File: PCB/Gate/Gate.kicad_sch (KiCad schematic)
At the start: 424 parts, among them J1 Conn_01x03, J2 Conn_01x03, U1 QR

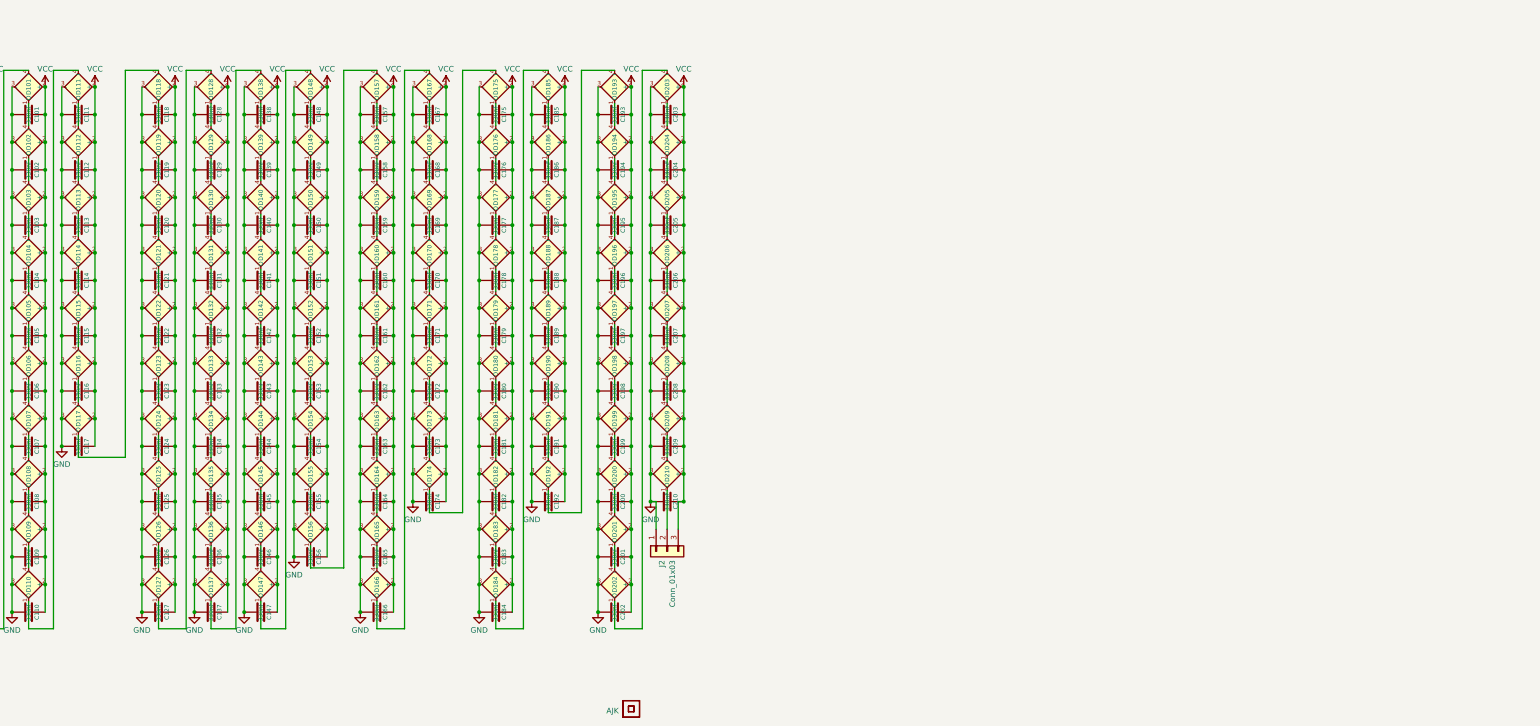
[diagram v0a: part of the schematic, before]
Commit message: Redone
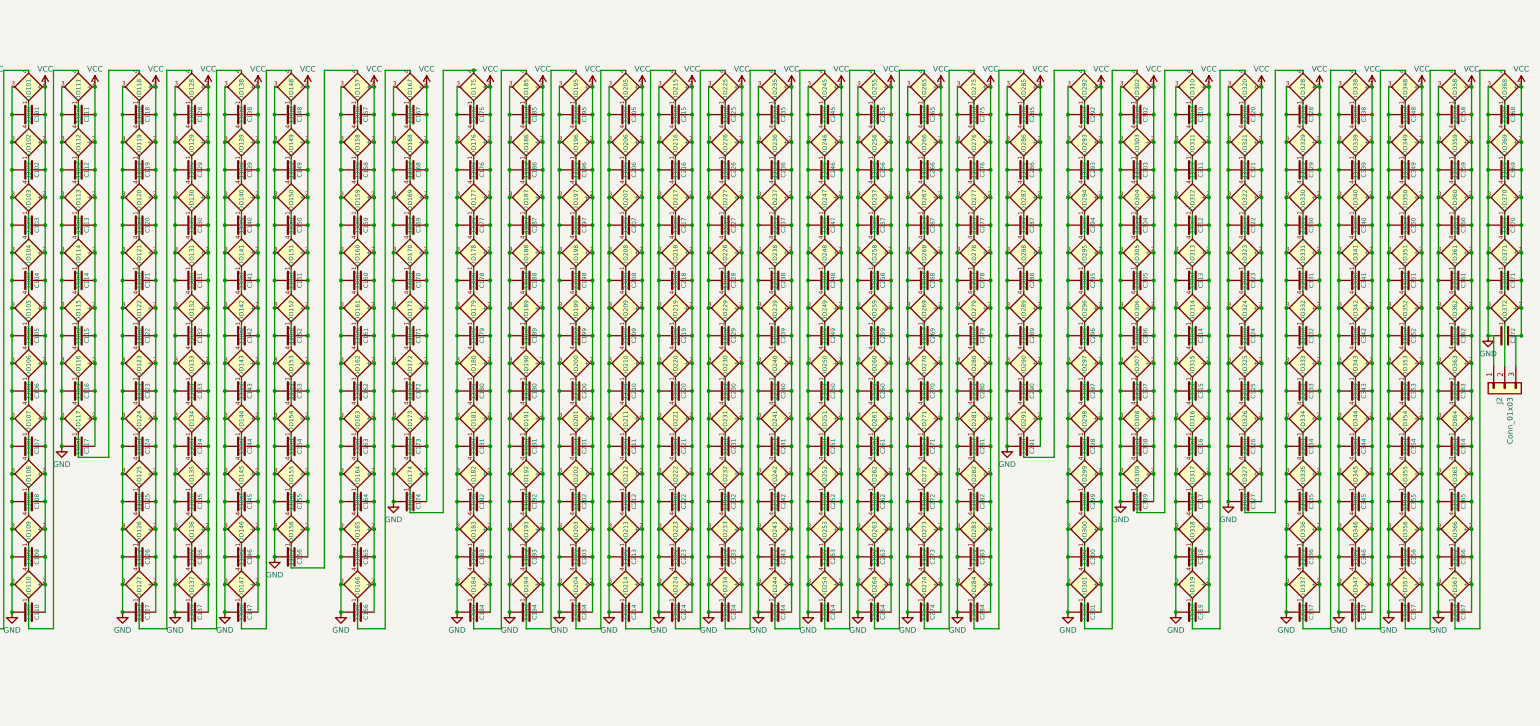
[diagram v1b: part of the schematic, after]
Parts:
- removed Logo1: AJK, RevK:AJK, symbol RevK:AJK
- removed U1: QR, RevK:QR-LED, symbol RevK:QR
- added C211, C212, C213, C214, C215, C216, C217, C218, C219, C220, C221, C222, C223, C224, C225, C226, C227, C228, C229, C230, C231, C232, C233, C234, C235, C236, C237, C238, C239, C240, C241, C242, C243, C244, C245, C246, C247, C248, C249, C250, C251, C252, C253, C254, C255, C256, C257, C258, C259, C260, C261, C262, C263, C264, C265, C266, C267, C268, C269, C270, C271, C272, C273, C274, C275, C276, C277, C278, C279, C280, C281, C282, C283, C284, C285, C286, C287, C288, C289, C290, C291, C292, C293, C294, C295, C296, C297, C298, C299, C300, C301, C302, C303, C304, C305, C306, C307, C308, C309, C310, C311, C312, C313, C314, C315, C316, C317, C318, C319, C320, C321, C322, C323, C324, C325, C326, C327, C328, C329, C330, C331, C332, C333, C334, C335, C336, C337, C338, C339, C340, C341, C342, C343, C344, C345, C346, C347, C348, C349, C350, C351, C352, C353, C354, C355, C356, C357, C358, C359, C360, C361, C362, C363, C364, C365, C366, C367, C368, C369, C370, C371, C372: 330nF, RevK:C_0402, symbol Device:C
- added D211, D212, D213, D214, D215, D216, D217, D218, D219, D220, D221, D222, D223, D224, D225, D226, D227, D228, D229, D230, D231, D232, D233, D234, D235, D236, D237, D238, D239, D240, D241, D242, D243, D244, D245, D246, D247, D248, D249, D250, D251, D252, D253, D254, D255, D256, D257, D258, D259, D260, D261, D262, D263, D264, D265, D266, D267, D268, D269, D270, D271, D272, D273, D274, D275, D276, D277, D278, D279, D280, D281, D282, D283, D284, D285, D286, D287, D288, D289, D290, D291, D292, D293, D294, D295, D296, D297, D298, D299, D300, D301, D302, D303, D304, D305, D306, D307, D308, D309, D310, D311, D312, D313, D314, D315, D316, D317, D318, D319, D320, D321, D322, D323, D324, D325, D326, D327, D328, D329, D330, D331, D332, D333, D334, D335, D336, D337, D338, D339, D340, D341, D342, D343, D344, D345, D346, D347, D348, D349, D350, D351, D352, D353, D354, D355, D356, D357, D358, D359, D360, D361, D362, D363, D364, D365, D366, D367, D368, D369, D370, D371, D372: XL-1010RGBC-WS2812B, RevK:SMD1010, symbol RevK:WS2812B-1mm
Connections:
- net GND: now also C211.2, C212.2, C213.2, C214.2, C215.2, C216.2, C217.2, C218.2, C219.2, C220.2, C221.2, C222.2, C223.2, C224.2, C225.2, C226.2, C227.2, C228.2, C229.2, C230.2, C231.2, C232.2, C233.2, C234.2, C235.2, C236.2, C237.2, C238.2, C239.2, C240.2, C241.2, C242.2, C243.2, C244.2, C245.2, C246.2, C247.2, C248.2, C249.2, C250.2, C251.2, C252.2, C253.2, C254.2, C255.2, C256.2, C257.2, C258.2, C259.2, C260.2, C261.2, C262.2, C263.2, C264.2, C265.2, C266.2, C267.2, C268.2, C269.2, C270.2, C271.2, C272.2, C273.2, C274.2, C275.2, C276.2, C277.2, C278.2, C279.2, C280.2, C281.2, C282.2, C283.2, C284.2, C285.2, C286.2, C287.2, C288.2, C289.2, C290.2, C291.2, C292.2, C293.2, C294.2, C295.2, C296.2, C297.2, C298.2, C299.2, C300.2, C301.2, C302.2, C303.2, C304.2, C305.2, C306.2, C307.2, C308.2, C309.2, C310.2, C311.2, C312.2, C313.2, C314.2, C315.2, C316.2, C317.2, C318.2, C319.2, C320.2, C321.2, C322.2, C323.2, C324.2, C325.2, C326.2, C327.2, C328.2, C329.2, C330.2, C331.2, C332.2, C333.2, C334.2, C335.2, C336.2, C337.2, C338.2, C339.2, C340.2, C341.2, C342.2, C343.2, C344.2, C345.2, C346.2, C347.2, C348.2, C349.2, C350.2, C351.2, C352.2, C353.2, C354.2, C355.2, C356.2, C357.2, C358.2, C359.2, C360.2, C361.2, C362.2, C363.2, C364.2, C365.2, C366.2, C367.2, C368.2, C369.2, C370.2, C371.2, C372.2, D211.3 (-), D212.3 (-), D213.3 (-), D214.3 (-), D215.3 (-), D216.3 (-), D217.3 (-), D218.3 (-), D219.3 (-), D220.3 (-), D221.3 (-), D222.3 (-), D223.3 (-), D224.3 (-), D225.3 (-), D226.3 (-), D227.3 (-), D228.3 (-), D229.3 (-), D230.3 (-), D231.3 (-), D232.3 (-), D233.3 (-), D234.3 (-), D235.3 (-), D236.3 (-), D237.3 (-), D238.3 (-), D239.3 (-), D240.3 (-), D241.3 (-), D242.3 (-), D243.3 (-), D244.3 (-), D245.3 (-), D246.3 (-), D247.3 (-), D248.3 (-), D249.3 (-), D250.3 (-), D251.3 (-), D252.3 (-), D253.3 (-), D254.3 (-), D255.3 (-), D256.3 (-), D257.3 (-), D258.3 (-), D259.3 (-), D260.3 (-), D261.3 (-), D262.3 (-), D263.3 (-), D264.3 (-), D265.3 (-), D266.3 (-), D267.3 (-), D268.3 (-), D269.3 (-), D270.3 (-), D271.3 (-), D272.3 (-), D273.3 (-), D274.3 (-), D275.3 (-), D276.3 (-), D277.3 (-), D278.3 (-), D279.3 (-), D280.3 (-), D281.3 (-), D282.3 (-), D283.3 (-), D284.3 (-), D285.3 (-), D286.3 (-), D287.3 (-), D288.3 (-), D289.3 (-), D290.3 (-), D291.3 (-), D292.3 (-), D293.3 (-), D294.3 (-), D295.3 (-), D296.3 (-), D297.3 (-), D298.3 (-), D299.3 (-), D300.3 (-), D301.3 (-), D302.3 (-), D303.3 (-), D304.3 (-), D305.3 (-), D306.3 (-), D307.3 (-), D308.3 (-), D309.3 (-), D310.3 (-), D311.3 (-), D312.3 (-), D313.3 (-), D314.3 (-), D315.3 (-), D316.3 (-), D317.3 (-), D318.3 (-), D319.3 (-), D320.3 (-), D321.3 (-), D322.3 (-), D323.3 (-), D324.3 (-), D325.3 (-), D326.3 (-), D327.3 (-), D328.3 (-), D329.3 (-), D330.3 (-), D331.3 (-), D332.3 (-), D333.3 (-), D334.3 (-), D335.3 (-), D336.3 (-), D337.3 (-), D338.3 (-), D339.3 (-), D340.3 (-), D341.3 (-), D342.3 (-), D343.3 (-), D344.3 (-), D345.3 (-), D346.3 (-), D347.3 (-), D348.3 (-), D349.3 (-), D350.3 (-), D351.3 (-), D352.3 (-), D353.3 (-), D354.3 (-), D355.3 (-), D356.3 (-), D357.3 (-), D358.3 (-), D359.3 (-), D360.3 (-), D361.3 (-), D362.3 (-), D363.3 (-), D364.3 (-), D365.3 (-), D366.3 (-), D367.3 (-), D368.3 (-), D369.3 (-), D370.3 (-), D371.3 (-), D372.3 (-)
- net VCC: now also C211.1, C212.1, C213.1, C214.1, C215.1, C216.1, C217.1, C218.1, C219.1, C220.1, C221.1, C222.1, C223.1, C224.1, C225.1, C226.1, C227.1, C228.1, C229.1, C230.1, C231.1, C232.1, C233.1, C234.1, C235.1, C236.1, C237.1, C238.1, C239.1, C240.1, C241.1, C242.1, C243.1, C244.1, C245.1, C246.1, C247.1, C248.1, C249.1, C250.1, C251.1, C252.1, C253.1, C254.1, C255.1, C256.1, C257.1, C258.1, C259.1, C260.1, C261.1, C262.1, C263.1, C264.1, C265.1, C266.1, C267.1, C268.1, C269.1, C270.1, C271.1, C272.1, C273.1, C274.1, C275.1, C276.1, C277.1, C278.1, C279.1, C280.1, C281.1, C282.1, C283.1, C284.1, C285.1, C286.1, C287.1, C288.1, C289.1, C290.1, C291.1, C292.1, C293.1, C294.1, C295.1, C296.1, C297.1, C298.1, C299.1, C300.1, C301.1, C302.1, C303.1, C304.1, C305.1, C306.1, C307.1, C308.1, C309.1, C310.1, C311.1, C312.1, C313.1, C314.1, C315.1, C316.1, C317.1, C318.1, C319.1, C320.1, C321.1, C322.1, C323.1, C324.1, C325.1, C326.1, C327.1, C328.1, C329.1, C330.1, C331.1, C332.1, C333.1, C334.1, C335.1, C336.1, C337.1, C338.1, C339.1, C340.1, C341.1, C342.1, C343.1, C344.1, C345.1, C346.1, C347.1, C348.1, C349.1, C350.1, C351.1, C352.1, C353.1, C354.1, C355.1, C356.1, C357.1, C358.1, C359.1, C360.1, C361.1, C362.1, C363.1, C364.1, C365.1, C366.1, C367.1, C368.1, C369.1, C370.1, C371.1, C372.1, D211.2 (+), D212.2 (+), D213.2 (+), D214.2 (+), D215.2 (+), D216.2 (+), D217.2 (+), D218.2 (+), D219.2 (+), D220.2 (+), D221.2 (+), D222.2 (+), D223.2 (+), D224.2 (+), D225.2 (+), D226.2 (+), D227.2 (+), D228.2 (+), D229.2 (+), D230.2 (+), D231.2 (+), D232.2 (+), D233.2 (+), D234.2 (+), D235.2 (+), D236.2 (+), D237.2 (+), D238.2 (+), D239.2 (+), D240.2 (+), D241.2 (+), D242.2 (+), D243.2 (+), D244.2 (+), D245.2 (+), D246.2 (+), D247.2 (+), D248.2 (+), D249.2 (+), D250.2 (+), D251.2 (+), D252.2 (+), D253.2 (+), D254.2 (+), D255.2 (+), D256.2 (+), D257.2 (+), D258.2 (+), D259.2 (+), D260.2 (+), D261.2 (+), D262.2 (+), D263.2 (+), D264.2 (+), D265.2 (+), D266.2 (+), D267.2 (+), D268.2 (+), D269.2 (+), D270.2 (+), D271.2 (+), D272.2 (+), D273.2 (+), D274.2 (+), D275.2 (+), D276.2 (+), D277.2 (+), D278.2 (+), D279.2 (+), D280.2 (+), D281.2 (+), D282.2 (+), D283.2 (+), D284.2 (+), D285.2 (+), D286.2 (+), D287.2 (+), D288.2 (+), D289.2 (+), D290.2 (+), D291.2 (+), D292.2 (+), D293.2 (+), D294.2 (+), D295.2 (+), D296.2 (+), D297.2 (+), D298.2 (+), D299.2 (+), D300.2 (+), D301.2 (+), D302.2 (+), D303.2 (+), D304.2 (+), D305.2 (+), D306.2 (+), D307.2 (+), D308.2 (+), D309.2 (+), D310.2 (+), D311.2 (+), D312.2 (+), D313.2 (+), D314.2 (+), D315.2 (+), D316.2 (+), D317.2 (+), D318.2 (+), D319.2 (+), D320.2 (+), D321.2 (+), D322.2 (+), D323.2 (+), D324.2 (+), D325.2 (+), D326.2 (+), D327.2 (+), D328.2 (+), D329.2 (+), D330.2 (+), D331.2 (+), D332.2 (+), D333.2 (+), D334.2 (+), D335.2 (+), D336.2 (+), D337.2 (+), D338.2 (+), D339.2 (+), D340.2 (+), D341.2 (+), D342.2 (+), D343.2 (+), D344.2 (+), D345.2 (+), D346.2 (+), D347.2 (+), D348.2 (+), D349.2 (+), D350.2 (+), D351.2 (+), D352.2 (+), D353.2 (+), D354.2 (+), D355.2 (+), D356.2 (+), D357.2 (+), D358.2 (+), D359.2 (+), D360.2 (+), D361.2 (+), D362.2 (+), D363.2 (+), D364.2 (+), D365.2 (+), D366.2 (+), D367.2 (+), D368.2 (+), D369.2 (+), D370.2 (+), D371.2 (+), D372.2 (+)
- net at D210.1 (O): now also D211.4 (I); no longer J2.2 (Pin_2)
- new net: D263.1 (O), D264.4 (I)
- new net: D262.1 (O), D263.4 (I)
- new net: D287.1 (O), D288.4 (I)
- new net: D286.1 (O), D287.4 (I)
- new net: D364.1 (O), D365.4 (I)
- new net: D363.1 (O), D364.4 (I)
- new net: D308.1 (O), D309.4 (I)
- new net: D307.1 (O), D308.4 (I)
- new net: D347.1 (O), D348.4 (I)
- new net: D346.1 (O), D347.4 (I)
- new net: D326.1 (O), D327.4 (I)
- new net: D325.1 (O), D326.4 (I)
- new net: D305.1 (O), D306.4 (I)
- new net: D304.1 (O), D305.4 (I)
- new net: D352.1 (O), D353.4 (I)
- new net: D351.1 (O), D352.4 (I)
- new net: D324.1 (O), D325.4 (I)
- new net: D294.1 (O), D295.4 (I)
- new net: D293.1 (O), D294.4 (I)
- new net: D296.1 (O), D297.4 (I)
- new net: D295.1 (O), D296.4 (I)
- new net: D271.1 (O), D272.4 (I)
- new net: D270.1 (O), D271.4 (I)
- new net: D244.1 (O), D245.4 (I)
- new net: D243.1 (O), D244.4 (I)
- new net: D261.1 (O), D262.4 (I)
- new net: D246.1 (O), D247.4 (I)
- new net: D245.1 (O), D246.4 (I)
- new net: D371.1 (O), D372.4 (I)
- new net: D370.1 (O), D371.4 (I)
- new net: D257.1 (O), D258.4 (I)
- new net: D256.1 (O), D257.4 (I)
- new net: D330.1 (O), D331.4 (I)
- new net: D329.1 (O), D330.4 (I)
- new net: D231.1 (O), D232.4 (I)
- new net: D230.1 (O), D231.4 (I)
- new net: D312.1 (O), D313.4 (I)
- new net: D311.1 (O), D312.4 (I)
- new net: D247.1 (O), D248.4 (I)
- new net: D260.1 (O), D261.4 (I)
- new net: D240.1 (O), D241.4 (I)
- new net: D239.1 (O), D240.4 (I)
- new net: D282.1 (O), D283.4 (I)
- new net: D281.1 (O), D282.4 (I)
- new net: D328.1 (O), D329.4 (I)
- new net: D253.1 (O), D254.4 (I)
- new net: D252.1 (O), D253.4 (I)
- new net: D251.1 (O), D252.4 (I)
- new net: D249.1 (O), D250.4 (I)
- new net: D248.1 (O), D249.4 (I)
- new net: D269.1 (O), D270.4 (I)
- new net: D280.1 (O), D281.4 (I)
- new net: D279.1 (O), D280.4 (I)
- new net: D290.1 (O), D291.4 (I)
- new net: D289.1 (O), D290.4 (I)
- new net: D356.1 (O), D357.4 (I)
- new net: D355.1 (O), D356.4 (I)
- new net: D342.1 (O), D343.4 (I)
- new net: D341.1 (O), D342.4 (I)
- new net: D278.1 (O), D279.4 (I)
- new net: D277.1 (O), D278.4 (I)
- new net: D338.1 (O), D339.4 (I)
- new net: D337.1 (O), D338.4 (I)
- new net: D228.1 (O), D229.4 (I)
- new net: D227.1 (O), D228.4 (I)
- new net: D259.1 (O), D260.4 (I)
- new net: D331.1 (O), D332.4 (I)
- new net: D224.1 (O), D225.4 (I)
- new net: D223.1 (O), D224.4 (I)
- new net: D310.1 (O), D311.4 (I)
- new net: D300.1 (O), D301.4 (I)
- new net: D299.1 (O), D300.4 (I)
- new net: D242.1 (O), D243.4 (I)
- new net: D241.1 (O), D242.4 (I)
- new net: D211.1 (O), D212.4 (I)
- new net: D336.1 (O), D337.4 (I)
- new net: D335.1 (O), D336.4 (I)
- new net: D372.1 (O), J2.2 (Pin_2)
- new net: D250.1 (O), D251.4 (I)
- new net: D362.1 (O), D363.4 (I)
- new net: D327.1 (O), D328.4 (I)
- new net: D229.1 (O), D230.4 (I)
- new net: D258.1 (O), D259.4 (I)
- new net: D369.1 (O), D370.4 (I)
- new net: D368.1 (O), D369.4 (I)
- new net: D268.1 (O), D269.4 (I)
- new net: D267.1 (O), D268.4 (I)
- new net: D234.1 (O), D235.4 (I)
- new net: D233.1 (O), D234.4 (I)
- new net: D212.1 (O), D213.4 (I)
- new net: D285.1 (O), D286.4 (I)
- new net: D284.1 (O), D285.4 (I)
- new net: D343.1 (O), D344.4 (I)
- new net: D288.1 (O), D289.4 (I)
- new net: D349.1 (O), D350.4 (I)
- new net: D348.1 (O), D349.4 (I)
- new net: D320.1 (O), D321.4 (I)
- new net: D319.1 (O), D320.4 (I)
- new net: D350.1 (O), D351.4 (I)
- new net: D353.1 (O), D354.4 (I)
- new net: D354.1 (O), D355.4 (I)
- new net: D298.1 (O), D299.4 (I)
- new net: D297.1 (O), D298.4 (I)
- new net: D323.1 (O), D324.4 (I)
- new net: D322.1 (O), D323.4 (I)
- new net: D345.1 (O), D346.4 (I)
- new net: D344.1 (O), D345.4 (I)
- new net: D266.1 (O), D267.4 (I)
- new net: D265.1 (O), D266.4 (I)
- new net: D216.1 (O), D217.4 (I)
- new net: D215.1 (O), D216.4 (I)
- new net: D360.1 (O), D361.4 (I)
- new net: D359.1 (O), D360.4 (I)
- new net: D291.1 (O), D292.4 (I)
- new net: D361.1 (O), D362.4 (I)
- new net: D232.1 (O), D233.4 (I)
- new net: D222.1 (O), D223.4 (I)
- new net: D221.1 (O), D222.4 (I)
- new net: D321.1 (O), D322.4 (I)
- new net: D217.1 (O), D218.4 (I)
- new net: D255.1 (O), D256.4 (I)
- new net: D226.1 (O), D227.4 (I)
- new net: D225.1 (O), D226.4 (I)
- new net: D301.1 (O), D302.4 (I)
- new net: D264.1 (O), D265.4 (I)
- new net: D275.1 (O), D276.4 (I)
- new net: D274.1 (O), D275.4 (I)
- new net: D276.1 (O), D277.4 (I)
- new net: D306.1 (O), D307.4 (I)
- new net: D332.1 (O), D333.4 (I)
- new net: D238.1 (O), D239.4 (I)
- new net: D237.1 (O), D238.4 (I)
- new net: D314.1 (O), D315.4 (I)
- new net: D313.1 (O), D314.4 (I)
- new net: D339.1 (O), D340.4 (I)
- new net: D254.1 (O), D255.4 (I)
- new net: D333.1 (O), D334.4 (I)
- new net: D309.1 (O), D310.4 (I)
- new net: D340.1 (O), D341.4 (I)
- new net: D317.1 (O), D318.4 (I)
- new net: D316.1 (O), D317.4 (I)
- new net: D365.1 (O), D366.4 (I)
- new net: D273.1 (O), D274.4 (I)
- new net: D272.1 (O), D273.4 (I)
- new net: D358.1 (O), D359.4 (I)
- new net: D357.1 (O), D358.4 (I)
- new net: D236.1 (O), D237.4 (I)
- new net: D235.1 (O), D236.4 (I)
- new net: D214.1 (O), D215.4 (I)
- new net: D218.1 (O), D219.4 (I)
- new net: D315.1 (O), D316.4 (I)
- new net: D292.1 (O), D293.4 (I)
- new net: D213.1 (O), D214.4 (I)
- new net: D334.1 (O), D335.4 (I)
- new net: D367.1 (O), D368.4 (I)
- new net: D302.1 (O), D303.4 (I)
- new net: D283.1 (O), D284.4 (I)
- new net: D303.1 (O), D304.4 (I)
- new net: D219.1 (O), D220.4 (I)
- new net: D366.1 (O), D367.4 (I)
- new net: D220.1 (O), D221.4 (I)
- new net: D318.1 (O), D319.4 (I)
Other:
- moved on the sheet: J2

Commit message: Cap value
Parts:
- C1, C10, C100, C101, C102, C103, C104, C105, C106, C107, C108, C109, C11, C110, C111, C112, C113, C114, C115, C116, C117, C118, C119, C12, C120, C121, C122, C123, C124, C125, C126, C127, C128, C129, C13, C130, C131, C132, C133, C134, C135, C136, C137, C138, C139, C14, C140, C141, C142, C143, C144, C145, C146, C147, C148, C149, C15, C150, C151, C152, C153, C154, C155, C156, C157, C158, C159, C16, C160, C161, C162, C163, C164, C165, C166, C167, C168, C169, C17, C170, C171, C172, C173, C174, C175, C176, C177, C178, C179, C18, C180, C181, C182, C183, C184, C185, C186, C187, C188, C189, C19, C190, C191, C192, C193, C194, C195, C196, C197, C198, C199, C2, C20, C200, C201, C202, C203, C204, C205, C206, C207, C208, C209, C21, C210, C211, C212, C213, C214, C215, C216, C217, C218, C219, C22, C220, C221, C222, C223, C224, C225, C226, C227, C228, C229, C23, C230, C231, C232, C233, C234, C235, C236, C237, C238, C239, C24, C240, C241, C242, C243, C244, C245, C246, C247, C248, C249, C25, C250, C251, C252, C253, C254, C255, C256, C257, C258, C259, C26, C260, C261, C262, C263, C264, C265, C266, C267, C268, C269, C27, C270, C271, C272, C273, C274, C275, C276, C277, C278, C279, C28, C280, C281, C282, C283, C284, C285, C286, C287, C288, C289, C29, C290, C291, C292, C293, C294, C295, C296, C297, C298, C299, C3, C30, C300, C301, C302, C303, C304, C305, C306, C307, C308, C309, C31, C310, C311, C312, C313, C314, C315, C316, C317, C318, C319, C32, C320, C321, C322, C323, C324, C325, C326, C327, C328, C329, C33, C330, C331, C332, C333, C334, C335, C336, C337, C338, C339, C34, C340, C341, C342, C343, C344, C345, C346, C347, C348, C349, C35, C350, C351, C352, C353, C354, C355, C356, C357, C358, C359, C36, C360, C361, C362, C363, C364, C365, C366, C367, C368, C369, C37, C370, C371, C372, C38, C39, C4, C40, C41, C42, C43, C44, C45, C46, C47, C48, C49, C5, C50, C51, C52, C53, C54, C55, C56, C57, C58, C59, C6, C60, C61, C62, C63, C64, C65, C66, C67, C68, C69, C7, C70, C71, C72, C73, C74, C75, C76, C77, C78, C79, C8, C80, C81, C82, C83, C84, C85, C86, C87, C88, C89, C9, C90, C91, C92, C93, C94, C95, C96, C97, C98, C99: value 330nF -> 100nF
